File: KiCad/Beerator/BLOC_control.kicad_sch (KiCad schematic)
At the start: 1 part

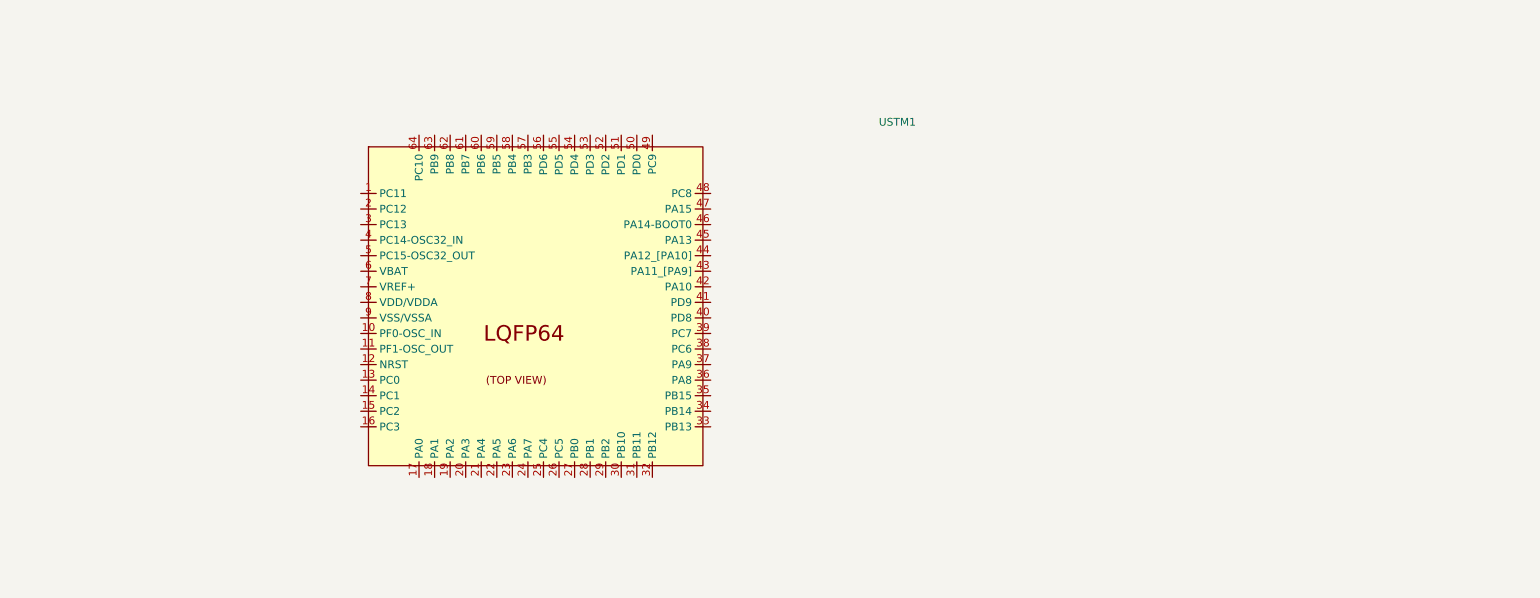
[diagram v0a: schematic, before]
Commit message: feat(Kicad): Schemas V1
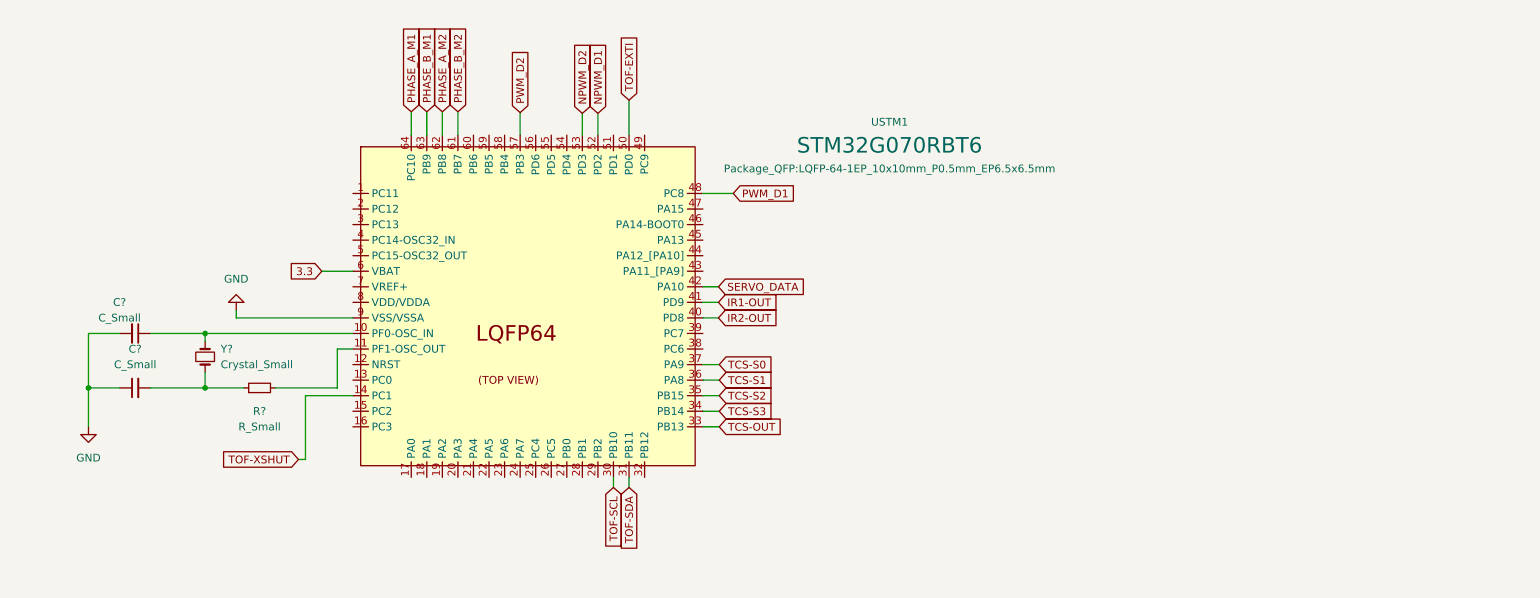
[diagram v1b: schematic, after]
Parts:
- added C? (x2): C_Small, symbol Device:C_Small
- added R?: R_Small, symbol Device:R_Small
- added Y?: Crystal_Small, symbol Device:Crystal_Small
- USTM1: value (none) -> STM32G070RBT6; footprint (none) -> Package_QFP:LQFP-64-1EP_10x10mm_P0.5mm_EP6.5x6.5mm
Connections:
- net at USTM1.10 (PF0-OSC_IN): now also C?.1, Y?.2
- net at USTM1.11 (PF1-OSC_OUT): now also R?.2
- net TOF-XSHUT: now reaches USTM1.14 (PC1)
- net TOF-SCL: now reaches USTM1.30 (PB10)
- net TOF-SDA: now reaches USTM1.31 (PB11)
- net TCS-OUT: now reaches USTM1.33 (PB13)
- net TCS-S3: now reaches USTM1.34 (PB14)
- net TCS-S2: now reaches USTM1.35 (PB15)
- net TCS-S1: now reaches USTM1.36 (PA8)
- net TCS-S0: now reaches USTM1.37 (PA9)
- net IR2-OUT: now reaches USTM1.40 (PD8)
- net IR1-OUT: now reaches USTM1.41 (PD9)
- net SERVO_DATA: now reaches USTM1.42 (PA10)
- net PWM_D1: now reaches USTM1.48 (PC8)
- net TOF-EXTI: now reaches USTM1.50 (PD0)
- net NPWM_D1: now reaches USTM1.52 (PD2)
- net NPWM_D2: now reaches USTM1.53 (PD3)
- net PWM_D2: now reaches USTM1.57 (PB3)
- net 3.3: now reaches USTM1.6 (VBAT)
- net PHASE_B_M2: now reaches USTM1.61 (PB7)
- net PHASE_A_M2: now reaches USTM1.62 (PB8)
- net PHASE_B_M1: now reaches USTM1.63 (PB9)
- net PHASE_A_M1: now reaches USTM1.64 (PC10)
- net GND: now reaches USTM1.9 (VSS/VSSA)
- net GND: now also C?.1, C?.2
- new net: C?.2, R?.1, Y?.1
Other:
- moved on the sheet: USTM1

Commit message: feat(KiCad): Version 2
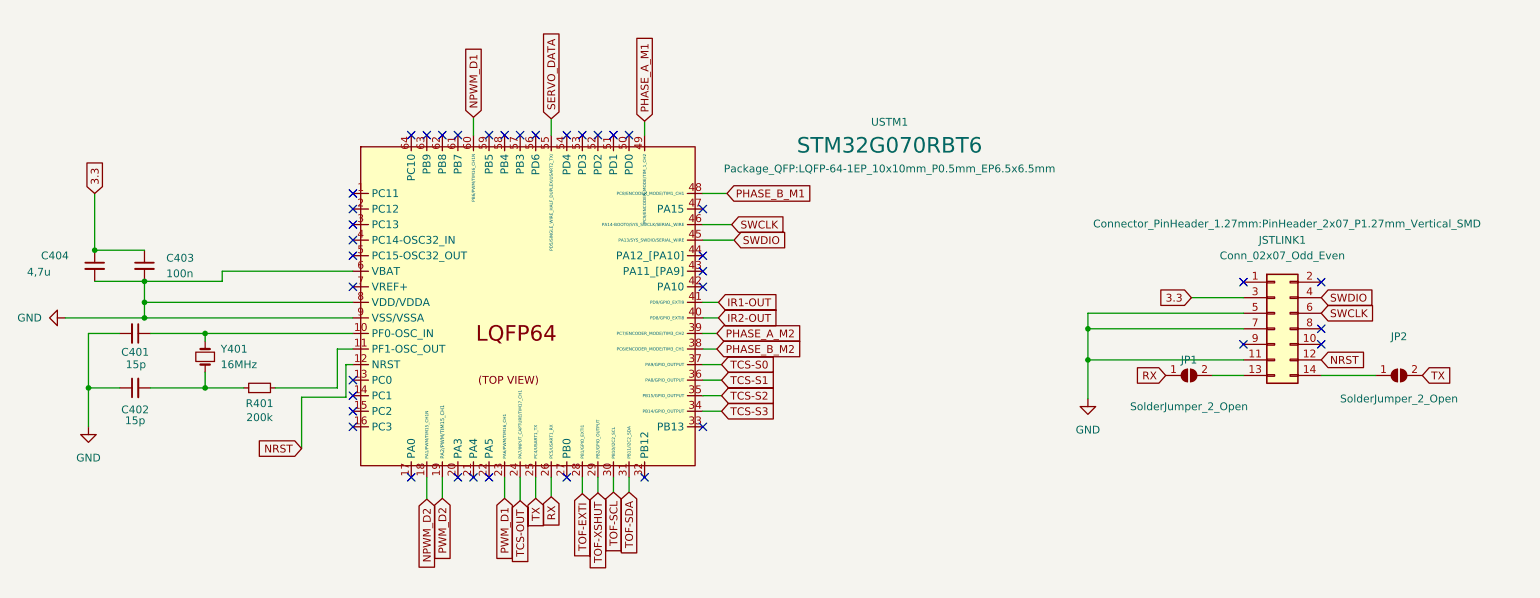
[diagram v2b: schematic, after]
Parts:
- added C403: 100n, symbol Device:C_Small
- added C404: 4,7u, symbol Device:C_Small
- added JP1, JP2: SolderJumper_2_Open, symbol Jumper:SolderJumper_2_Open
- added JSTLINK1: Conn_02x07_Odd_Even, Connector_PinHeader_1.27mm:PinHeader_2x07_P1.27mm_Vertical_SMD, symbol Connector_Generic:Conn_02x07_Odd_Even
- C401, C402: renamed from C?; value C_Small -> 15p
- R401: renamed from R?; value R_Small -> 200k
- Y401: renamed from Y?; value Crystal_Small -> 16MHz
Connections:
- net 3.3: now also C403.1, C404.1, JSTLINK1.3 (Pin_3); no longer USTM1.6 (VBAT)
- net GND: now also USTM1.6 (VBAT), USTM1.8 (VDD/VDDA), C403.2, C404.2, JSTLINK1.11 (Pin_11), JSTLINK1.5 (Pin_5), JSTLINK1.7 (Pin_7)
- net NPWM_D1: now also USTM1.60 (PB6/PWM/TIM16_CH1N); no longer USTM1.52 (PD2)
- net NPWM_D2: now also USTM1.18 (PA1/PWM/TIM15_CH1N); no longer USTM1.53 (PD3)
- net PHASE_A_M1: now also USTM1.49 (PC9/ENCODER_MODE/TIM_1_CH2); no longer USTM1.64 (PC10)
- net PHASE_A_M2: now also USTM1.39 (PC7/ENCODER_MODE/TIM3_CH2); no longer USTM1.62 (PB8)
- net PHASE_B_M1: now also USTM1.48 (PC8/ENCODER_MODE/TIM1_CH1); no longer USTM1.63 (PB9)
- net PHASE_B_M2: now also USTM1.38 (PC6/ENCODER_MODE/TIM3_CH1); no longer USTM1.61 (PB7)
- net PWM_D1: now also USTM1.23 (PA6/PWM/TIM16_CH1); no longer USTM1.48 (PC8)
- net PWM_D2: now also USTM1.19 (PA2/PWM/TIM15_CH1); no longer USTM1.57 (PB3)
- net SERVO_DATA: now also USTM1.55 (PD5/SINGLE_WIRE_HALF_DUPLEX/USART2_TX/); no longer USTM1.42 (PA10)
- net TCS-OUT: now also USTM1.24 (PA7/INPUT_CAPTURE/TIM17_CH1); no longer USTM1.33 (PB13)
- net TOF-EXTI: now also USTM1.28 (PB1/GPIO_EXTI1); no longer USTM1.50 (PD0)
- net TOF-XSHUT: now also USTM1.29 (PB2/GPIO_OUTPUT); no longer USTM1.14 (PC1)
- net NRST: now reaches USTM1.12 (NRST)
- net NRST: now also JSTLINK1.12 (Pin_12)
- net TX: now reaches USTM1.25 (PC4/USART1_TX)
- net TX: now also JP2.2 (B)
- net RX: now reaches USTM1.26 (PC5/USART1_RX)
- net RX: now also JP1.1 (A)
- net SWDIO: now reaches USTM1.45 (PA13/SYS_SWDIO/SERIAL_WIRE)
- net SWDIO: now also JSTLINK1.4 (Pin_4)
- net SWCLK: now reaches USTM1.46 (PA14-BOOT0/SYS_SWCLK/SERIAL_WIRE)
- net SWCLK: now also JSTLINK1.6 (Pin_6)
- new net: JP2.1 (A), JSTLINK1.14 (Pin_14)
- new net: JP1.2 (B), JSTLINK1.13 (Pin_13)
- no-connect marks 0 -> 39
